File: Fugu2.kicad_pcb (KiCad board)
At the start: 2 copper layers, 50 x 88 mm, 128 parts, among them J10 691256610002, J2 I2C Conn, J3 Conn_L_SW, J4 MCU head, J5 UART (CAN) Conn, J6 Conn_L_out, J7 3.3V PSU, J9 691256610002, P2 QTGM027, Q1 IPA050N10NM5S, Q2 IPP022N12NM6, Q3 IPA050N10NM5S, Q4 BSS123, Q5 TPH1R306PL,L1Q or NTMFS5C612N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, Q6 TPH1R306PL,L1Q or NTMFS5C612N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, Q7 TPH1R306PL,L1Q or NTMFS5C612N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, Q8 GT800N10D3, Q9 BSS123, SW1 SW_Push, U1 UCC21330BQDRQ1, U2 ESP32-S3-WROOM-1-N4, U3 INA226, U5 AP3012

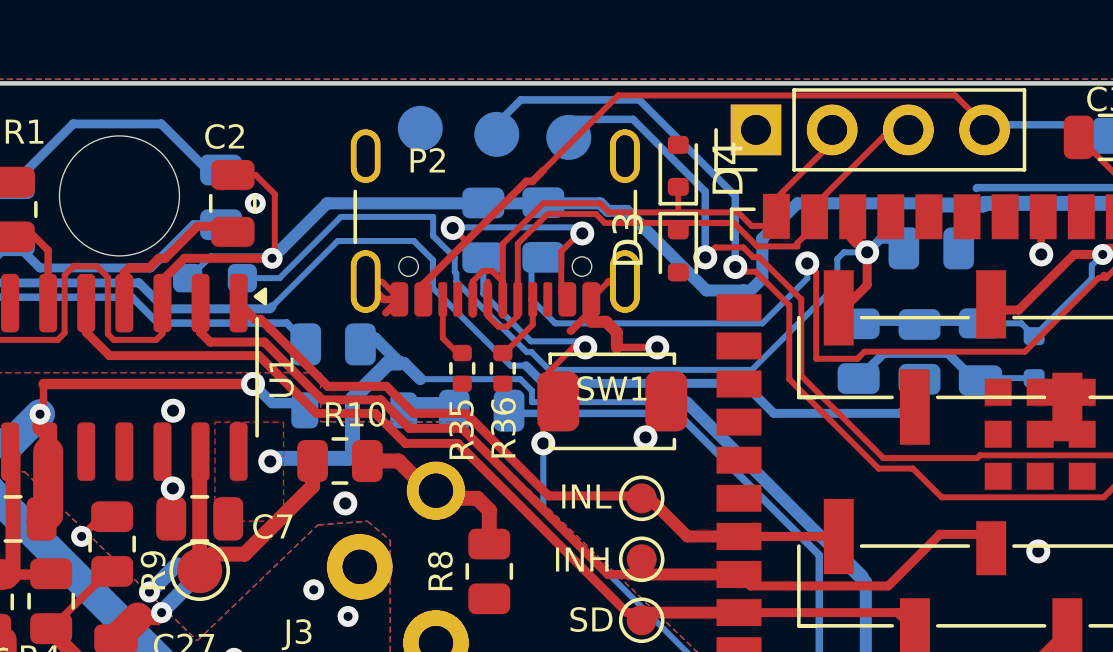
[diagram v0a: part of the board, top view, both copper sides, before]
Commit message: Add RC connection between USB-C shield and GND
1. Added a 1 MΩ resistor and 10 nF capacitor between the USB Type-C connector shield and GND in the schematic and PCB layout.
2. Added clearer USB connector symbol having no missing pads
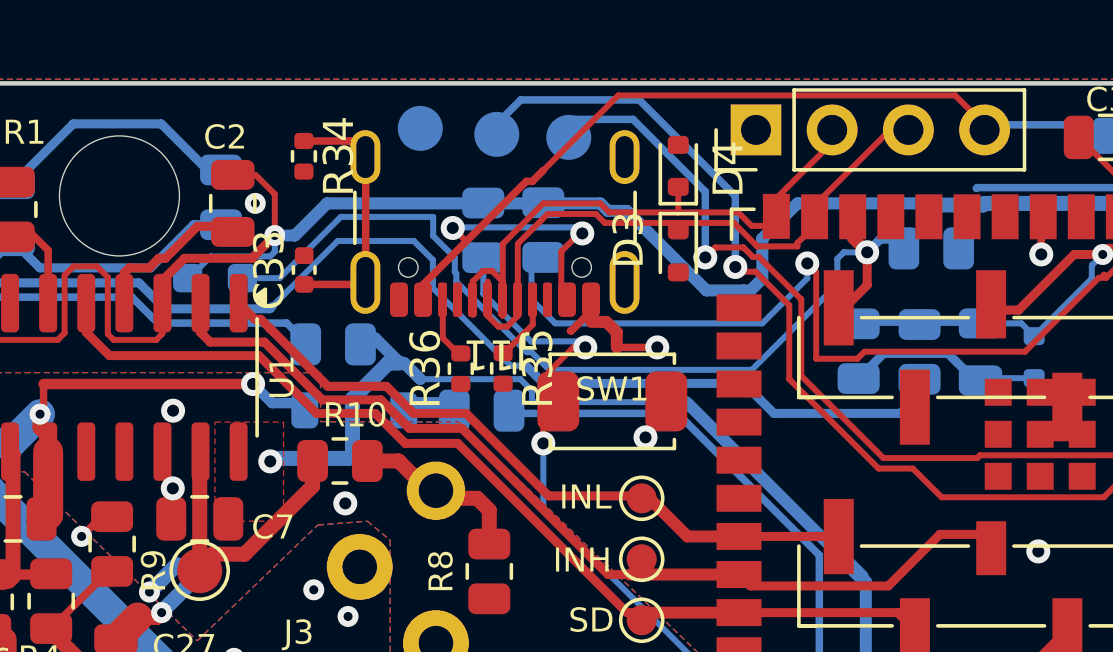
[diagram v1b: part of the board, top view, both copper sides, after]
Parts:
- removed P2: QTGM027, open-pe:USB_C_Receptacle_GCT_USB4105-xx-A_16P_TopMnt_Horizontal
- added C33: 10n, Capacitor_SMD:C_0402_1005Metric, F.Cu at (44.6, 37.2)
- added J11: QTGM027, Library:USB_C_Receptacle_GCT_USB4105-xx-A_16P_TopMnt_Horizontal, F.Cu at (51.0, 34.5)
- added R34: 1M, Resistor_SMD:R_0402_1005Metric, F.Cu at (44.6, 33.4)
- R35, R36: value 5.1k 1% -> 5.1k
- moved R36 1.40 mm to (49.9, 40.5), turned to 90 degrees
- moved R35 1.36 mm to (51.3, 40.5)
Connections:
- R36 pad 1: Net-(P2-CC) -> GND
- R36 pad 2: GND -> Net-(J11-CC2)
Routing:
- net Net-(J11-SHIELD): track 0.00 -> 8.48 mm
- net GND: track 126.4 -> 122.2 mm
- net Net-(P2-CC): track 2.12 -> 0.00 mm
- net Net-(J11-CC2): track 0.00 -> 2.02 mm
